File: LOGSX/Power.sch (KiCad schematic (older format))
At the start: 23 parts, among them IC2 STC3117IJT, J2 BATTERY CONN, J3 POWER IN, SW1 SW_SPDT, U2 LT1129-3.3_SO8, U3 MCP73113_4

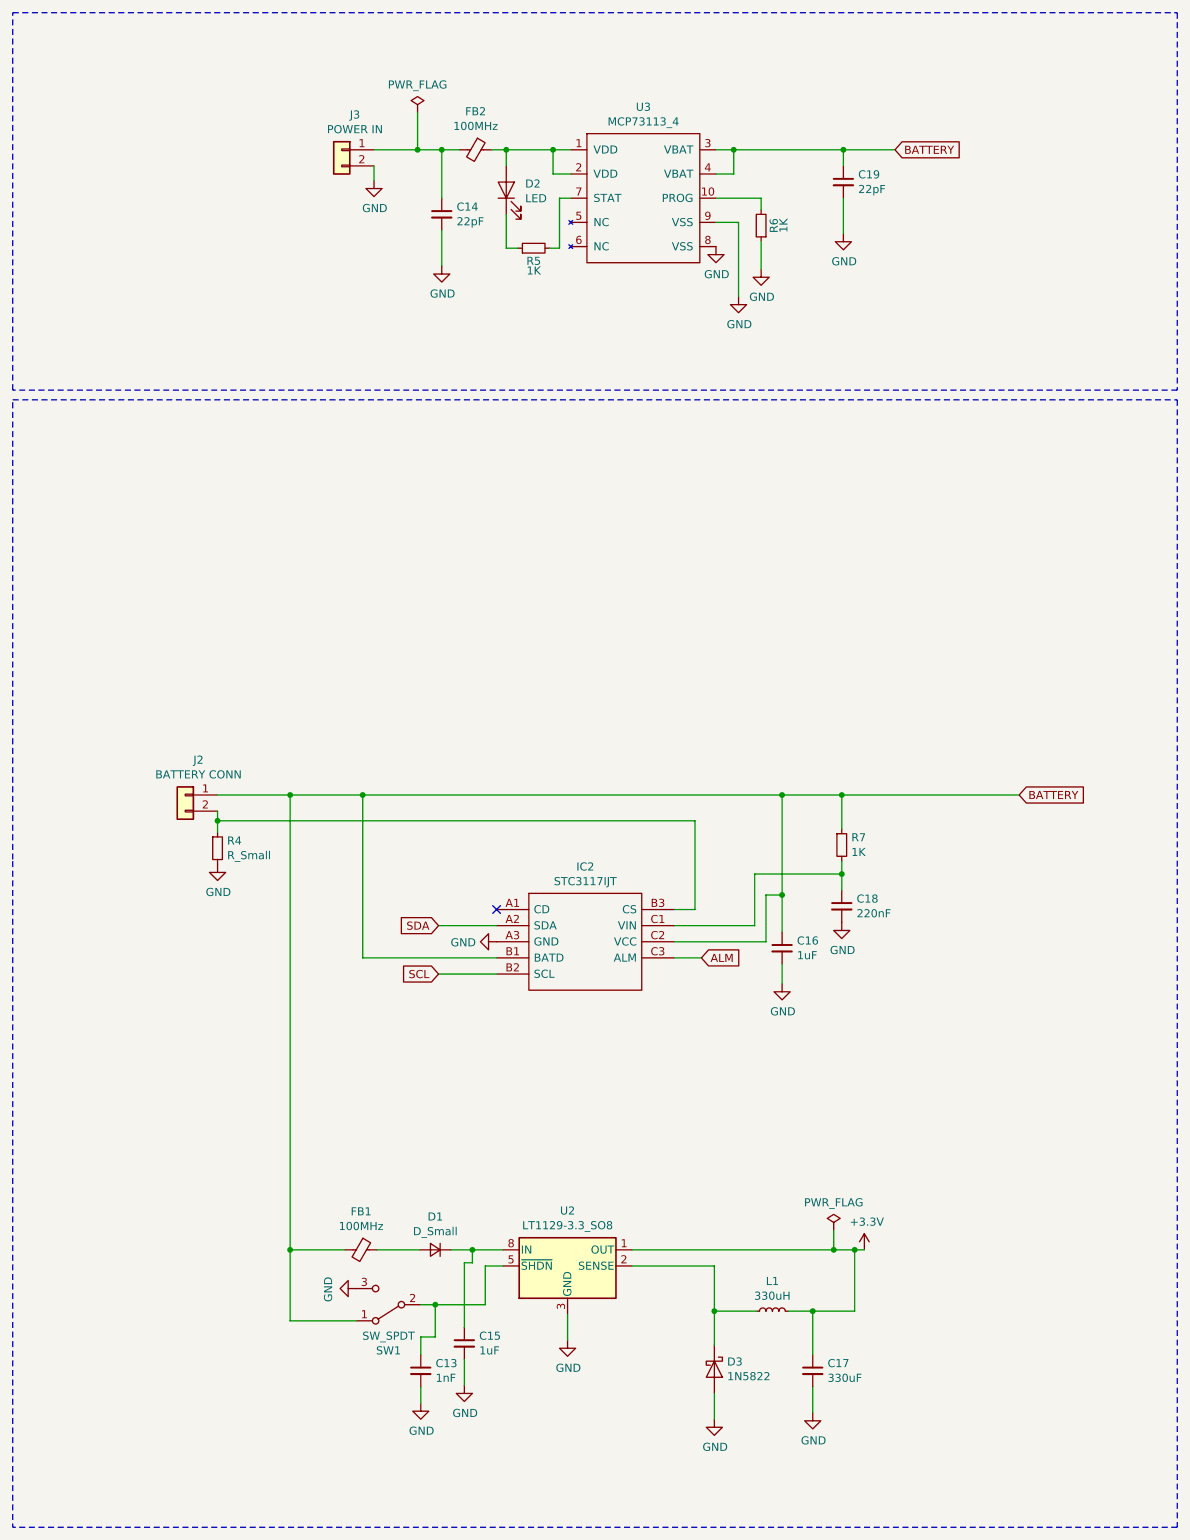
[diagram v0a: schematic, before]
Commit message: Add files via upload
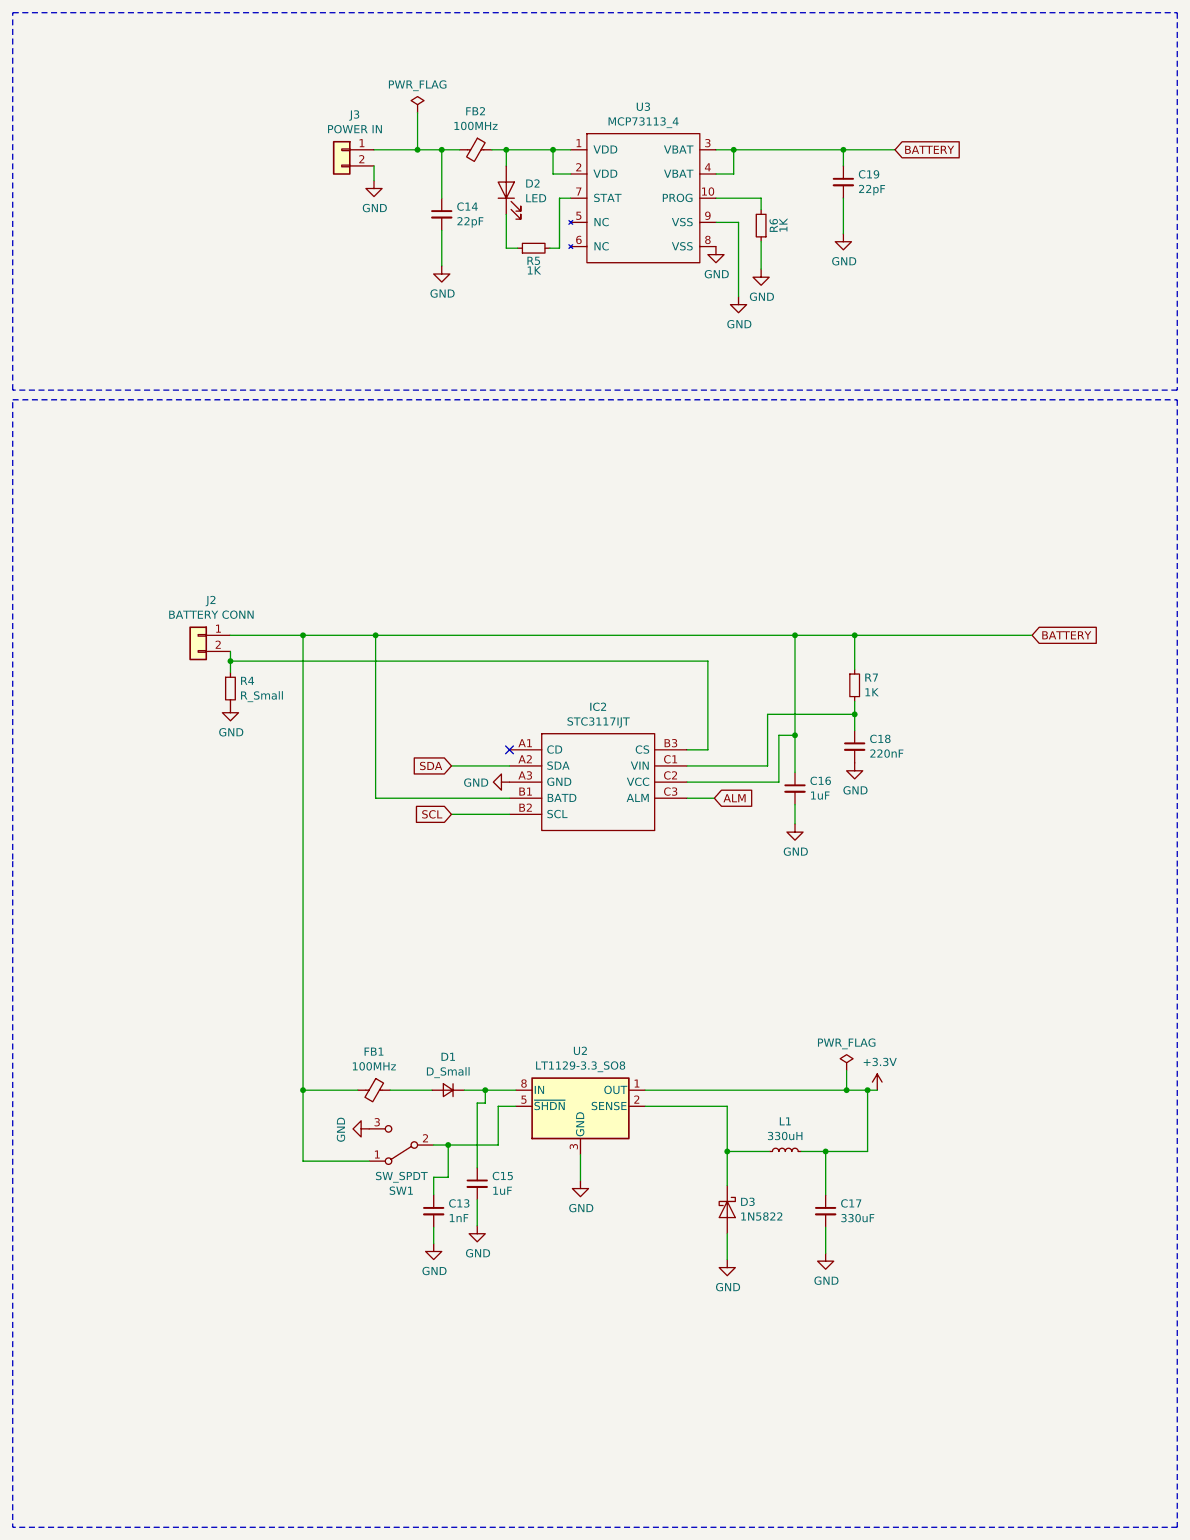
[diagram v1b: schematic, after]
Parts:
- D3: footprint Diode_THT:D_DO-201AD_P15.24mm_Horizontal -> Diode_SMD:D_0402_1005Metric
- J2: footprint Connector_JST:JST_PH_B2B-PH-SM4-TB_1x02-1MP_P2.00mm_Vertical -> Battery:BatteryHolder_Keystone_1042_1x18650
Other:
- moved on the sheet: C13, C15, C16, C17, C18, D1, D3, FB1, IC2, J2, L1, R4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

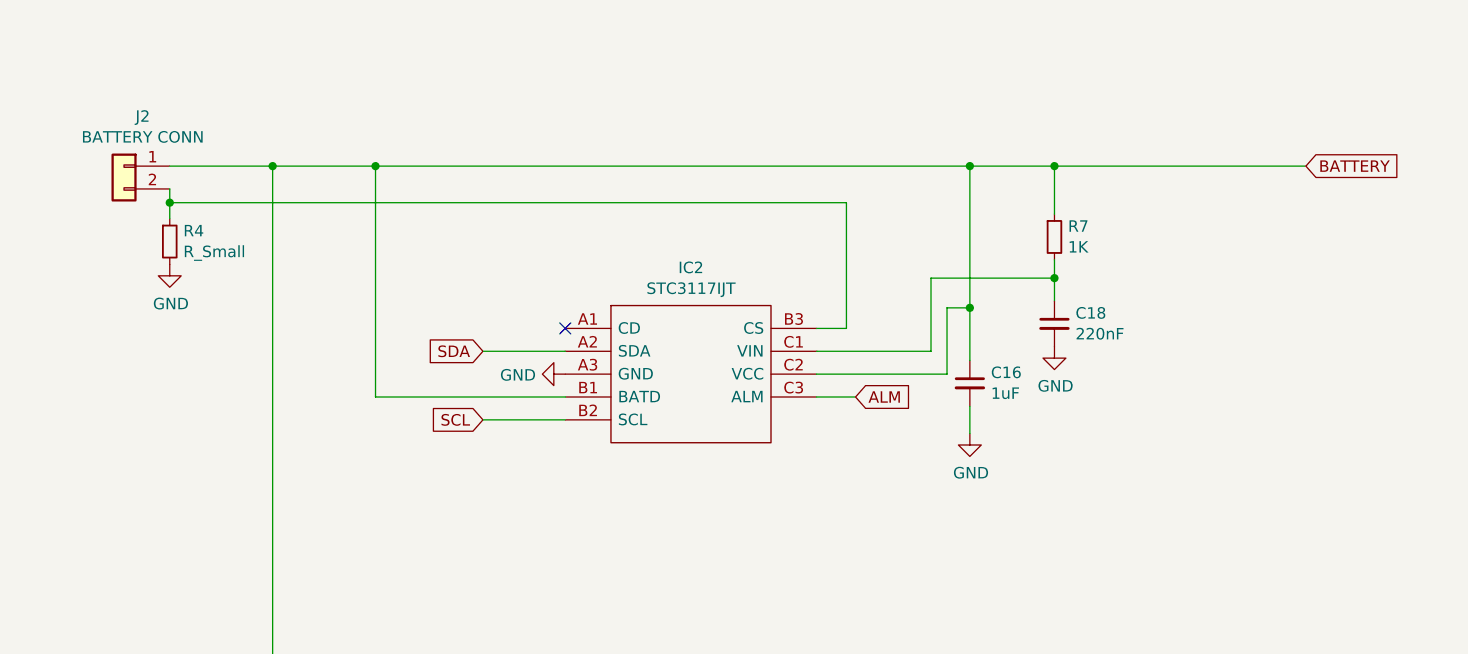
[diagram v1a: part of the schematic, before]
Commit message: Add files via upload
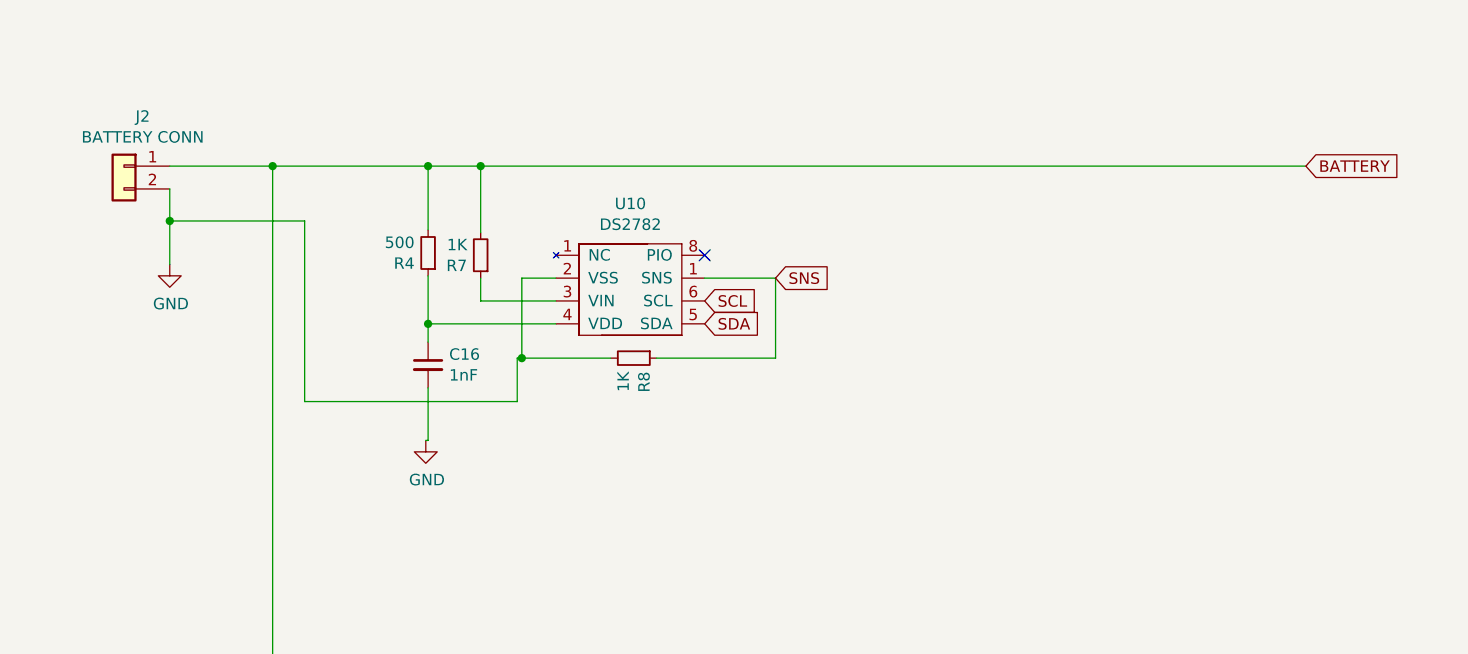
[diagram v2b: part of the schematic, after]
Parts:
- removed C18: 220nF, Capacitor_SMD:C_0402_1005Metric, symbol Device:C_Small
- removed IC2: STC3117IJT, ASSETS:BGA9C40P3X3_146X156X66, symbol Regular_Use:STC3117IJT
- added R8: 1K, Resistor_SMD:R_0402_1005Metric, symbol Device:R_Small
- added U10: DS2782, Package_SO:TSSOP-8_4.4x3mm_P0.65mm, symbol Regular_Use:DS2782
- C16: value 1uF -> 1nF; footprint Capacitor_SMD:C_0402_1005Metric -> Capacitor_SMD:C_0201_0603Metric
- R4: value R_Small -> 500
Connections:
- net BATTERY: now also R4.2, R7.2; no longer C16.1, R7.1
- net GND: now also J2.2 (Pin_2), R8.2, U10.2 (VSS); no longer R4.2
- net SCL: now also U10.6 (SCL)
- net SDA: now also U10.5 (SDA)
- net at R4.1: now also C16.1, U10.4 (VDD); no longer J2.2 (Pin_2)
- new net: R7.1, U10.3 (VIN)
- new net SNS: R8.1, U10.1 (SNS)
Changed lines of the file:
@@
 Wire Wire Line
 	3030 1370 3180 1370
-$Comp
-L Regular_Use:STC3117IJT IC2
-U 1 1 5EBFF472
-P 3600 5090
-F 0 "IC2" H 4150 5355 50  0000 C CNN
-F 1 "STC3117IJT" H 4150 5264 50  0000 C CNN
-F 2 "ASSETS:BGA9C40P3X3_146X156X66" H 4550 5190 50  0001 L CNN
-F 3 "https://componentsearchengine.com/Datasheets/1/STC3117IJT.pdf" H 4550 5090 50  0001 L CNN
-F 4 "Battery Management ANALOG" H 4550 4990 50  0001 L CNN "Description"
-F 5 "0.655" H 4550 4890 50  0001 L CNN "Height"
-F 6 "511-STC3117IJT" H 4550 4790 50  0001 L CNN "Mouser Part Number"
-F 7 "https://www.mouser.com/Search/Refine.aspx?Keyword=511-STC3117IJT" H 4550 4690 50  0001 L CNN "Mouser Price/Stock"
-F 8 "STMicroelectronics" H 4550 4590 50  0001 L CNN "Manufacturer_Name"
-F 9 "STC3117IJT" H 4550 4490 50  0001 L CNN "Manufacturer_Part_Number"
-	1    3600 5090
-	1    0    0    -1
-$EndComp
 Wire Wire Line
 	5670 1370 5990 1370
@@
 Wire Notes Line
 	520  520  7740 520
-NoConn ~ 3600 5090
-Wire Wire Line
-	3600 5190 3240 5190
-Text GLabel 3240 5190 0    50   Input ~ 0
-SDA
-$Comp
-L power:GND #PWR036
-U 1 1 5EC095C2
-P 3600 5290
-F 0 "#PWR036" H 3600 5040 50  0001 C CNN
-F 1 "GND" V 3605 5162 50  0000 R CNN
-F 2 "" H 3600 5290 50  0001 C CNN
-F 3 "" H 3600 5290 50  0001 C CNN
-	1    3600 5290
-	0    1    1    0
-$EndComp
-Wire Wire Line
-	3600 5490 3240 5490
-Text GLabel 3240 5490 0    50   Input ~ 0
-SCL
 $Comp
 L Connector_Generic:Conn_01x02 J2
@@
 	1    0    0    -1
 $EndComp
-$Comp
-L Device:R_Small R4
-U 1 1 5EC0DE7D
-P 1870 4710
-F 0 "R4" H 1929 4756 50  0000 L CNN
-F 1 "R_Small" H 1929 4665 50  0000 L CNN
-F 2 "Resistor_SMD:R_0402_1005Metric" H 1870 4710 50  0001 C CNN
-F 3 "~" H 1870 4710 50  0001 C CNN
-	1    1870 4710
-	1    0    0    -1
-$EndComp
-Wire Wire Line
-	1870 4480 1870 4540
-Wire Wire Line
-	4700 5090 4830 5090
-Wire Wire Line
-	4830 5090 4830 4540
-Wire Wire Line
-	4830 4540 1870 4540
-Connection ~ 1870 4540
-Wire Wire Line
-	1870 4540 1870 4610
-Wire Wire Line
-	2770 5390 2770 4380
-Wire Wire Line
-	2770 5390 3600 5390
-Connection ~ 2770 4380
-Wire Wire Line
-	2770 4380 5370 4380
-$Comp
-L Device:R_Small R7
-U 1 1 5EC11458
-P 5740 4690
-F 0 "R7" H 5799 4736 50  0000 L CNN
-F 1 "1K" H 5799 4645 50  0000 L CNN
-F 2 "Resistor_SMD:R_0402_1005Metric" H 5740 4690 50  0001 C CNN
-F 3 "~" H 5740 4690 50  0001 C CNN
-	1    5740 4690
-	1    0    0    -1
-$EndComp
-Wire Wire Line
-	5740 4590 5740 4380
-Connection ~ 5740 4380
-Wire Wire Line
-	5740 4380 6840 4380
-$Comp
-L Device:C_Small C18
-U 1 1 5EC12427
-P 5740 5070
-F 0 "C18" H 5832 5116 50  0000 L CNN
-F 1 "220nF" H 5832 5025 50  0000 L CNN
-F 2 "Capacitor_SMD:C_0402_1005Metric" H 5740 5070 50  0001 C CNN
-F 3 "~" H 5740 5070 50  0001 C CNN
-	1    5740 5070
-	1    0    0    -1
-$EndComp
-Wire Wire Line
-	5740 4790 5740 4870
-Wire Wire Line
-	4700 5190 5200 5190
-Wire Wire Line
-	5200 5190 5200 4870
-Wire Wire Line
-	5200 4870 5740 4870
-Connection ~ 5740 4870
-Wire Wire Line
-	5740 4870 5740 4970
-$Comp
-L power:GND #PWR044
-U 1 1 5EC1423C
-P 5740 5170
-F 0 "#PWR044" H 5740 4920 50  0001 C CNN
-F 1 "GND" H 5745 4997 50  0000 C CNN
-F 2 "" H 5740 5170 50  0001 C CNN
-F 3 "" H 5740 5170 50  0001 C CNN
-	1    5740 5170
-	1    0    0    -1
-$EndComp
-$Comp
-L Device:C_Small C16
-U 1 1 5EC14C8B
-P 5370 5330
-F 0 "C16" H 5462 5376 50  0000 L CNN
-F 1 "1uF" H 5462 5285 50  0000 L CNN
-F 2 "Capacitor_SMD:C_0402_1005Metric" H 5370 5330 50  0001 C CNN
-F 3 "~" H 5370 5330 50  0001 C CNN
-	1    5370 5330
-	1    0    0    -1
-$EndComp
-Wire Wire Line
-	5370 5230 5370 5000
-Connection ~ 5370 4380
-Wire Wire Line
-	5370 4380 5740 4380
-$Comp
-L power:GND #PWR042
-U 1 1 5EC16054
-P 5370 5550
-F 0 "#PWR042" H 5370 5300 50  0001 C CNN
-F 1 "GND" H 5375 5377 50  0000 C CNN
-F 2 "" H 5370 5550 50  0001 C CNN
-F 3 "" H 5370 5550 50  0001 C CNN
-	1    5370 5550
-	1    0    0    -1
-$EndComp
-Wire Wire Line
-	5370 5430 5370 5550
-Wire Wire Line
-	4700 5290 5270 5290
-Wire Wire Line
-	5270 5290 5270 5000
-Wire Wire Line
-	5270 5000 5370 5000
-Connection ~ 5370 5000
-Wire Wire Line
-	5370 5000 5370 4380
-Wire Wire Line
-	4700 5390 4870 5390
-Text GLabel 4870 5390 2    50   Input ~ 0
-ALM
 Wire Notes Line
 	520  2920 7740 2920
@@
 	2320 7200 2320 4380
 Connection ~ 2320 4380
-Wire Wire Line
-	2320 4380 2770 4380
 Wire Wire Line
 	3640 7300 3530 7300
@@
 Wire Wire Line
 	3130 8150 3130 8050
+$Comp
+L Regular_Use:DS2782 U10
+U 1 1 5EC1CB22
+P 3660 4720
+F 0 "U10" H 3885 4895 50  0000 C CNN
+F 1 "DS2782" H 3885 4804 50  0000 C CNN
+F 2 "Package_SO:TSSOP-8_4.4x3mm_P0.65mm" H 3660 4870 50  0001 C CNN
+F 3 "" H 3660 4870 50  0001 C CNN
+	1    3660 4720
+	1    0    0    -1
+$EndComp
+Text GLabel 4210 5070 2    50   Input ~ 0
+SDA
+Text GLabel 4210 4970 2    50   Input ~ 0
+SCL
+$Comp
+L Device:R_Small R8
+U 1 1 5EC1FF93
+P 3900 5220
+F 0 "R8" H 3959 5266 50  0000 L CNN
+F 1 "1K" H 3959 5175 50  0000 L CNN
+F 2 "Resistor_SMD:R_0402_1005Metric" H 3900 5220 50  0001 C CNN
+F 3 "~" H 3900 5220 50  0001 C CNN
+	1    3900 5220
+	0    1    1    0
+$EndComp
+Wire Wire Line
+	4210 4870 4520 4870
+Wire Wire Line
+	4520 4870 4520 5220
+Wire Wire Line
+	3560 4870 3410 4870
+Wire Wire Line
+	3410 4870 3410 5220
+Wire Wire Line
+	3410 5220 3800 5220
+NoConn ~ 4210 4770
+$Comp
+L Device:R_Small R7
+U 1 1 5EC28BAB
+P 3230 4770
+F 0 "R7" H 3289 4816 50  0000 L CNN
+F 1 "1K" H 3289 4725 50  0000 L CNN
+F 2 "Resistor_SMD:R_0402_1005Metric" H 3230 4770 50  0001 C CNN
+F 3 "~" H 3230 4770 50  0001 C CNN
+	1    3230 4770
+	-1   0    0    1
+$EndComp
+$Comp
+L Device:R_Small R4
+U 1 1 5EC28FB1
+P 3000 4760
+F 0 "R4" H 3059 4806 50  0000 L CNN
+F 1 "500" H 3059 4715 50  0000 L CNN
+F 2 "Resistor_SMD:R_0402_1005Metric" H 3000 4760 50  0001 C CNN
+F 3 "~" H 3000 4760 50  0001 C CNN
+	1    3000 4760
+	-1   0    0    1
+$EndComp
+Wire Wire Line
+	3560 4970 3230 4970
+Wire Wire Line
+	3230 4970 3230 4870
+Wire Wire Line
+	3560 5070 3000 5070
+Wire Wire Line
+	3000 5070 3000 4860
+Wire Wire Line
+	2320 4380 3000 4380
+Wire Wire Line
+	1870 4480 1870 4620
+Wire Wire Line
+	3000 4660 3000 4380
+Connection ~ 3000 4380
+Wire Wire Line
+	3000 4380 3230 4380
+Wire Wire Line
+	3230 4670 3230 4380
+Connection ~ 3230 4380
+Wire Wire Line
+	3230 4380 6840 4380
+$Comp
+L Device:C_Small C16
+U 1 1 5EC3C8A5
+P 3000 5250
+F 0 "C16" H 3092 5296 50  0000 L CNN
+F 1 "1nF" H 3092 5205 50  0000 L CNN
+F 2 "Capacitor_SMD:C_0201_0603Metric" H 3000 5250 50  0001 C CNN
+F 3 "~" H 3000 5250 50  0001 C CNN
+	1    3000 5250
+	1    0    0    -1
+$EndComp
+Wire Wire Line
+	3000 5150 3000 5070
+Connection ~ 3000 5070
+Wire Wire Line
+	3000 5350 3000 5580
+Wire Wire Line
+	3000 5580 2990 5580
+$Comp
+L power:GND #PWR05
+U 1 1 5EC41CD0
+P 2990 5580
+F 0 "#PWR05" H 2990 5330 50  0001 C CNN
+F 1 "GND" H 2995 5407 50  0000 C CNN
+F 2 "" H 2990 5580 50  0001 C CNN
+F 3 "" H 2990 5580 50  0001 C CNN
+	1    2990 5580
+	1    0    0    -1
+$EndComp
+Wire Wire Line
+	3410 5220 3390 5220
+Wire Wire Line
+	3390 5220 3390 5410
+Wire Wire Line
+	3390 5410 2460 5410
+Wire Wire Line
+	2460 5410 2460 4620
+Wire Wire Line
+	2460 4620 1870 4620
+Connection ~ 3410 5220
+Connection ~ 1870 4620
+Wire Wire Line
+	1870 4620 1870 4810
+Wire Wire Line
+	4000 5220 4520 5220
+Text GLabel 4520 4870 2    50   Input ~ 0
+SNS
 $EndSCHEMATC
